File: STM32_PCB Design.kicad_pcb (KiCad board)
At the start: 2 copper layers, 28 parts, among them J1 USB_B_Micro, J2 Conn_01x04_Pin, J3 Conn_01x04_Pin, J4 Conn_01x04_Pin, SW1 SW_SPDT, U1 STM32F103C8T6, U2 AMS1117-3.3, Y1 16MHz

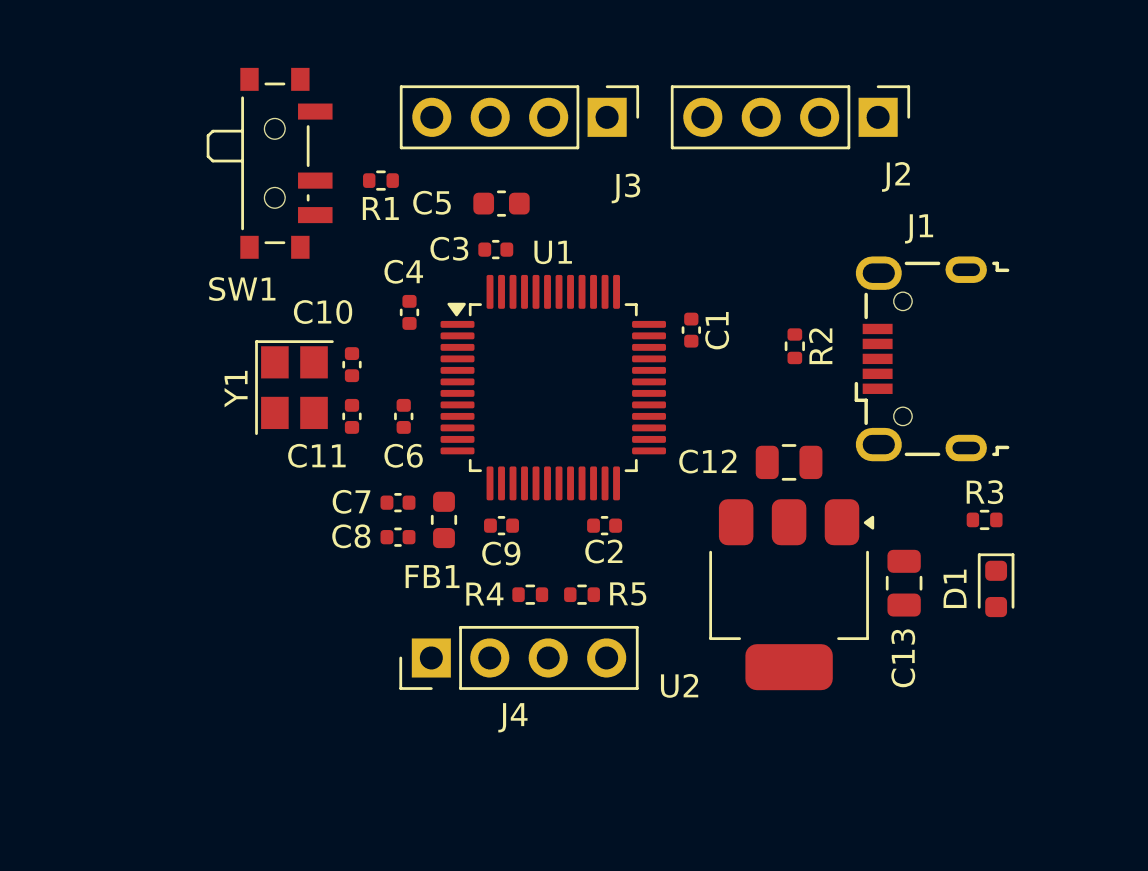
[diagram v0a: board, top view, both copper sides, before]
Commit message: Completed routing of components
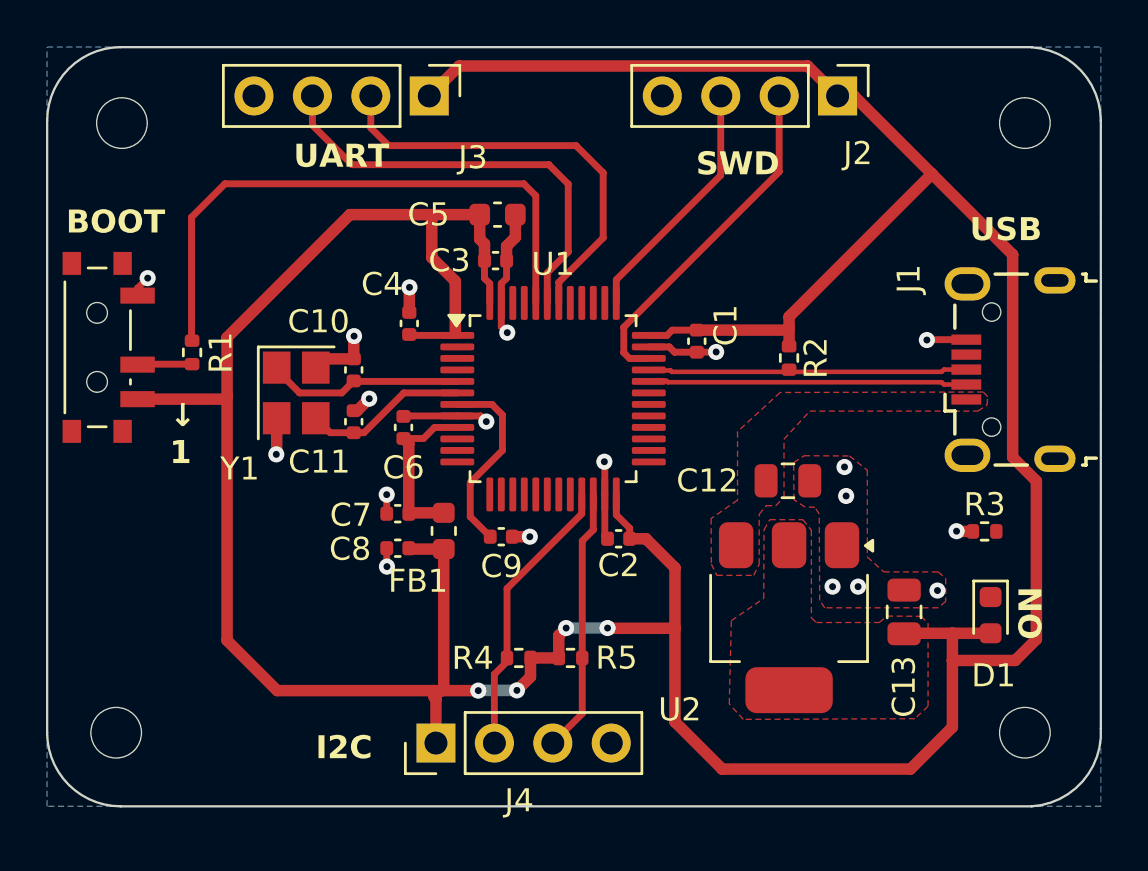
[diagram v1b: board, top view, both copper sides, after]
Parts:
- added H1: MountingHole, MountingHole:MountingHole_2.2mm_M2, F.Cu at (30.2, 29.5)
- added H2: MountingHole, MountingHole:MountingHole_2.2mm_M2, F.Cu at (69.5, 29.5)
- added H3: MountingHole, MountingHole:MountingHole_2.2mm_M2, F.Cu at (30.0, 56.0)
- added H4: MountingHole, MountingHole:MountingHole_2.2mm_M2, F.Cu at (69.5, 56.0)
- moved SW1 11.1 mm to (29.5, 39.2)
- moved R1 11.1 mm to (33.3, 39.5), turned to 90 degrees
- moved J3 7.79 mm to (43.6, 28.3)
- moved J1 3.88 mm to (68.9, 40.2)
- moved J4 3.71 mm to (43.9, 56.5)
- moved R4 2.80 mm to (47.5, 52.8)
- moved R5 2.80 mm to (49.8, 52.8)
- moved J2 1.99 mm to (61.4, 28.3)
- moved C13 1.25 mm to (64.2, 50.8)
- moved D1 1.16 mm to (68.0, 50.9)
- moved U2 1.00 mm to (59.2, 51.0)
- moved C2 0.83 mm to (51.8, 47.6)
- moved C12 0.80 mm to (59.2, 45.0)
- moved R2 0.57 mm to (59.2, 39.7)
- moved C1 0.54 mm to (55.2, 39.0)
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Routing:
- net +3.3V: track 0.00 -> 174.2 mm, vias 0 -> 4
- net GND: track 0.00 -> 27.8 mm, vias 0 -> 19
- net /BOOT0: track 0.00 -> 25.8 mm
- net /USART_RX: track 0.00 -> 19.0 mm
- net /USART_TX: track 0.00 -> 18.8 mm
- net /SWDIO: track 0.00 -> 15.2 mm
- net /USB_D-: track 0.00 -> 13.9 mm
- net /USB_D+: track 0.00 -> 13.9 mm
- net /I2C2_SCL: track 0.00 -> 12.4 mm
- net /I2C2_SDA: track 0.00 -> 11.5 mm
- net /SWCLK: track 0.00 -> 10.9 mm
- net /HSE__IN: track 0.00 -> 8.59 mm
- net /NRST: track 0.00 -> 8.39 mm
- net +3.3VA: track 0.00 -> 7.44 mm
- net /HSE_OUT: track 0.00 -> 7.13 mm
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- added copper zone on F.Cu, net +3.3V
- added copper zone on B.Cu, net GND
- added copper zone on F.Cu, net GND
- added copper zone on F.Cu, net VBUS
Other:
- board outline added: 45.8 x 33 mm
- board text added: "BOOT"
- board text added: "I2C"
- board text added: "ON"
- board text added: "SWD"
- board text added: "UART"
- board text added: "USB"
- board text added: "↓ 1"
